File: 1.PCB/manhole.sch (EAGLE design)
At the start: 21 parts, among them IC1 7805TV

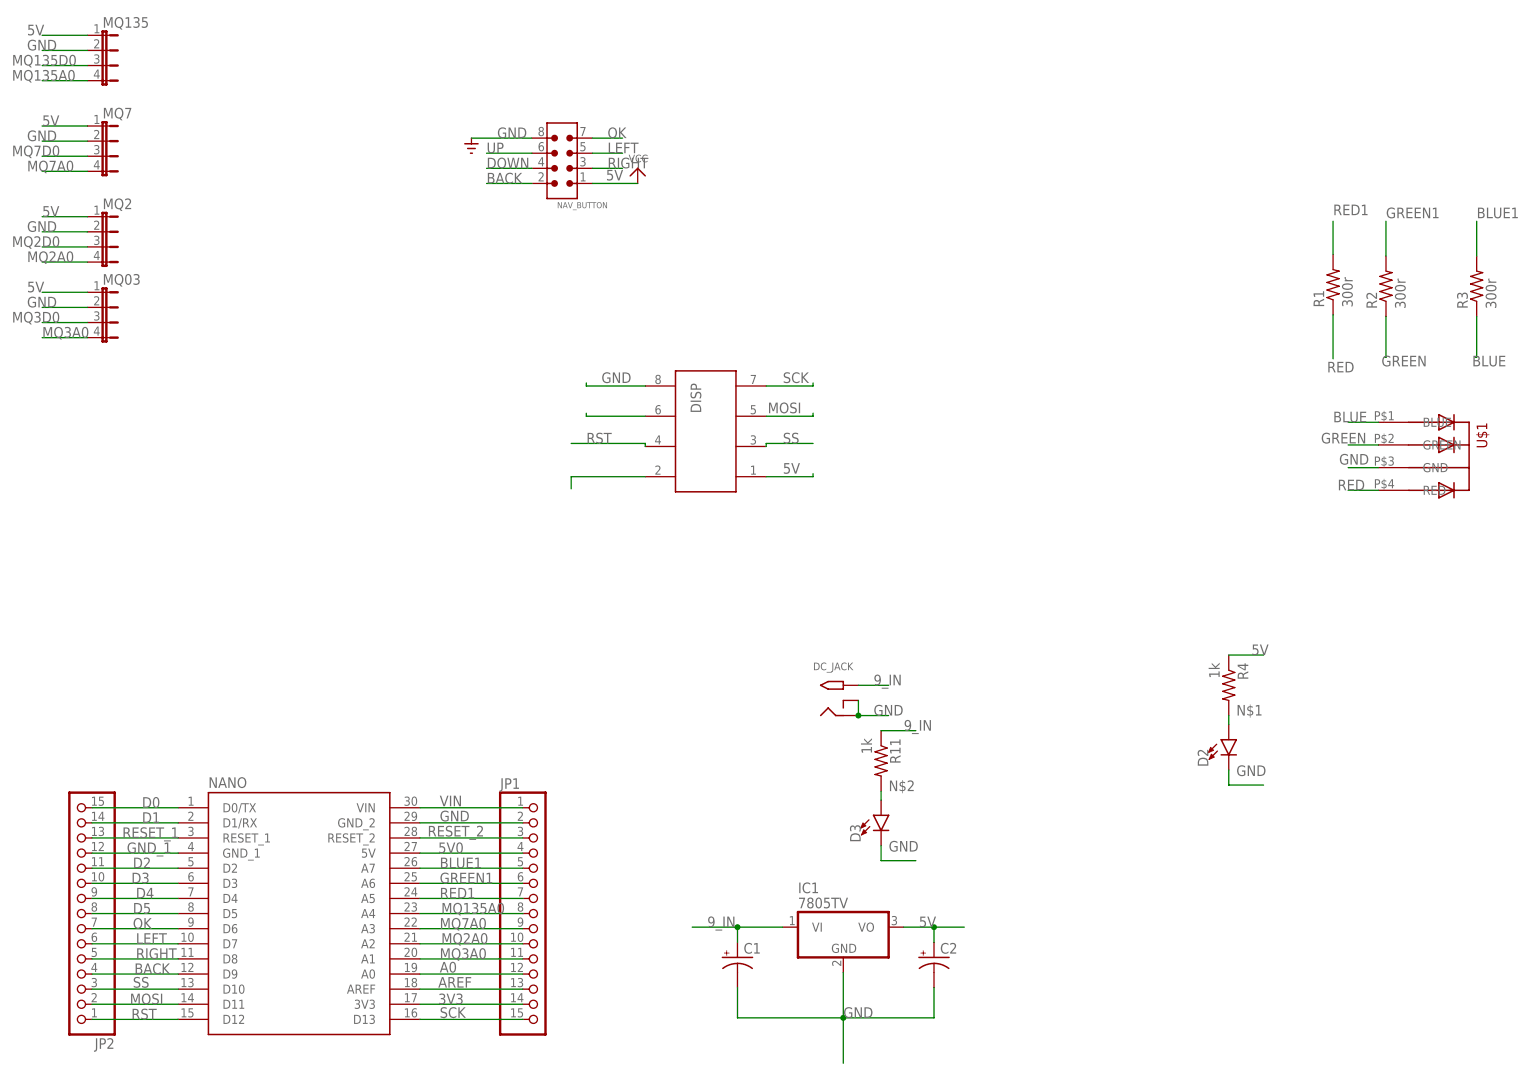
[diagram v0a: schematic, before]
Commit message: Add files via upload
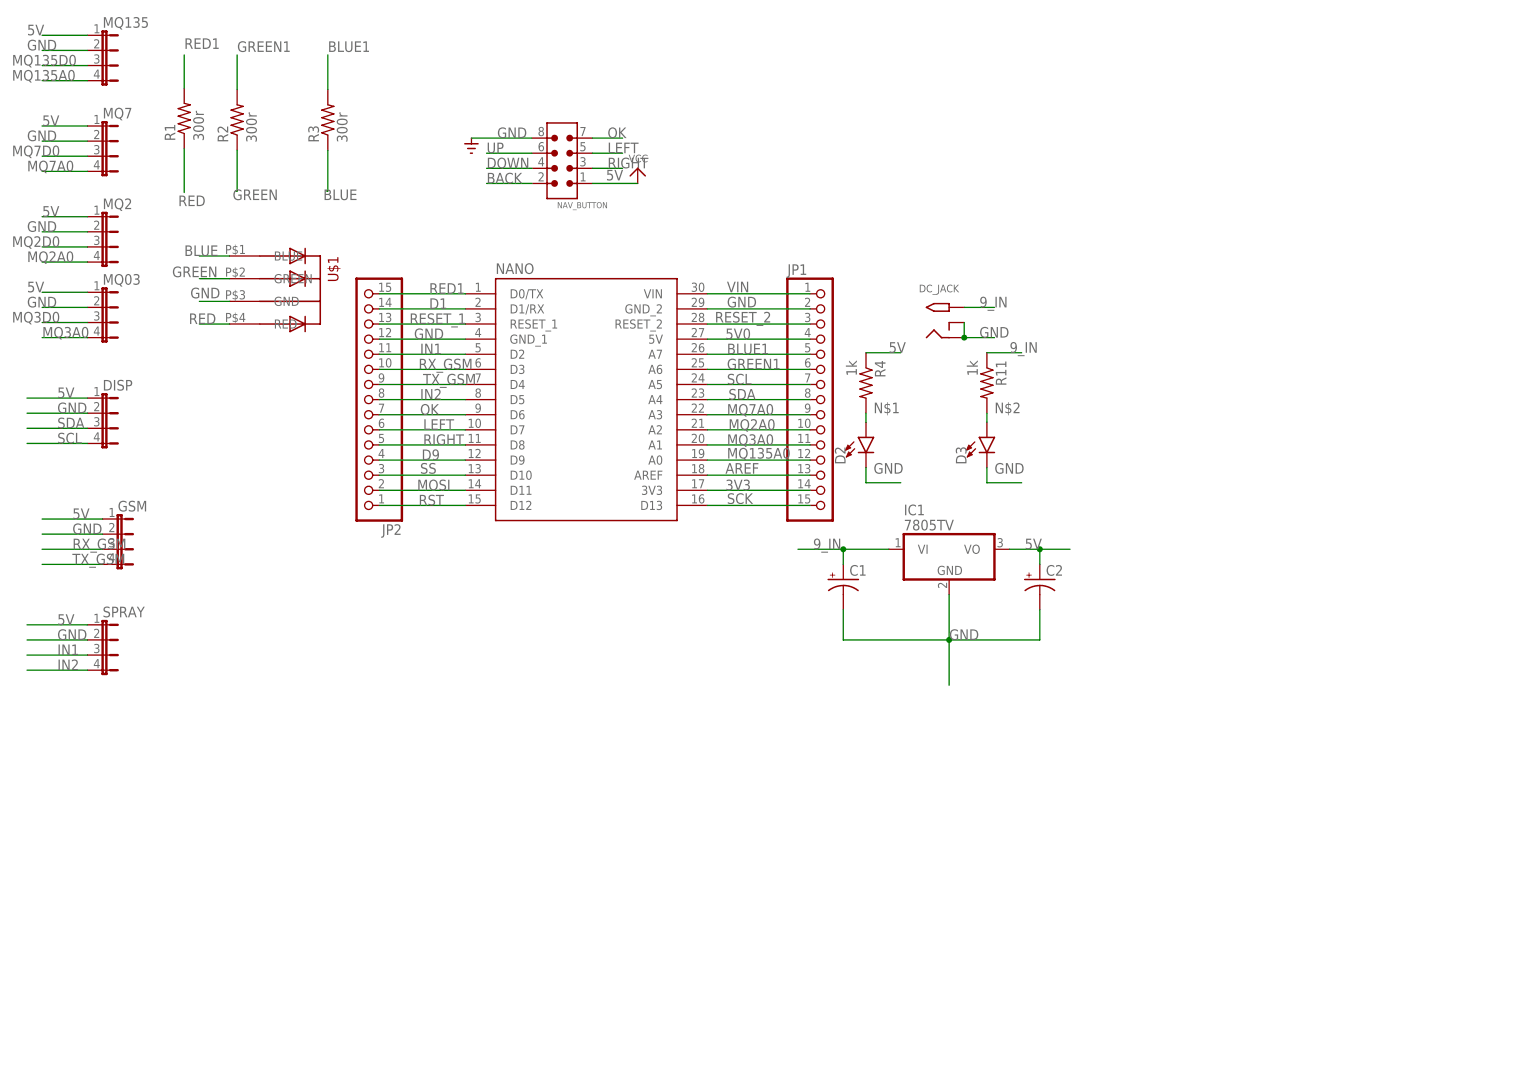
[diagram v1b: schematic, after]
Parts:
- added GSM, SPRAY: (no value), jumper:JP4E
- DISP: device Wurth_Elektronik_Electromechanic_Wire_to_Board_Connectors_rev19a:612008235121 -> jumper:JP4E
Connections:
- removed net A0: JP1.12, NANO.A0
- removed net D0: JP2.15, NANO.D0/TX
- removed net D2: JP2.11, NANO.D2
- removed net D3: JP2.10, NANO.D3
- removed net D4: JP2.9, NANO.D4
- removed net D5: JP2.8, NANO.D5
- removed net GND_1: JP2.12, NANO.GND_1
- removed net N$3: DISP.2
- removed net N$5: DISP.6
- new net D9: JP2.4, NANO.D9
- new net IN1: JP2.11, NANO.D2, SPRAY.3
- new net IN2: JP2.8, NANO.D5, SPRAY.4
- new net RX_GSM: GSM.3, JP2.10, NANO.D3
- new net SCL: DISP.4, JP1.7, NANO.A5
- new net SDA: DISP.3, JP1.8, NANO.A4
- new net TX_GSM: GSM.4, JP2.9, NANO.D4
- net 5V: now also GSM.1, SPRAY.1
- net BACK: no longer JP2.4, NANO.D9
- net GND: now also DISP.2, GSM.2, JP2.12, NANO.GND_1, SPRAY.2; no longer DISP.8
- net MOSI: no longer DISP.5
- net MQ135A0: now also JP1.12, NANO.A0; no longer JP1.8, NANO.A4
- net RED1: now also JP2.15, NANO.D0/TX; no longer JP1.7, NANO.A5
- net RST: no longer DISP.4
- net SCK: no longer DISP.7
- net SS: no longer DISP.3
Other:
- moved on the sheet: C1, C2, D2, D3, DC_JACK, IC1, JP1, JP2, NANO, R1, R11, R2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
